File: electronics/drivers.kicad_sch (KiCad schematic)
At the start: 37 parts, among them J10 Conn_01x02_Pin, J12 GND, J13 Conn_01x08_Pin, J14 IOLV / VIO, J8 VMOT, J9 BP_MOTOR_ENABLE, Q2 PMOS_GDS, U10 ISO7762DBQ, U11 LM1117DT-3.3, U12 SFH617A-1, U8 SFH617A-1, U9 74LVC125

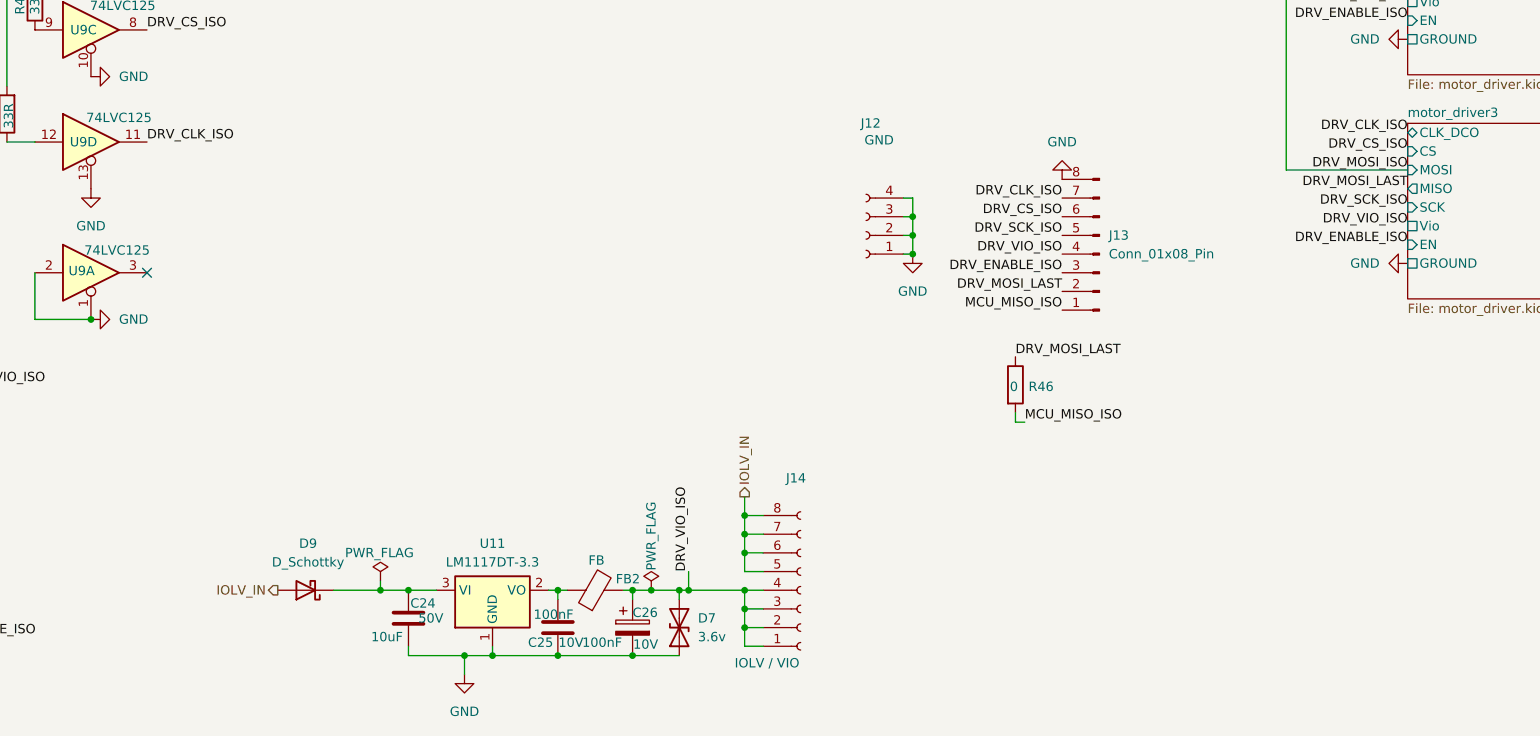
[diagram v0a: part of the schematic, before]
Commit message: Updating electronics CAD post-production
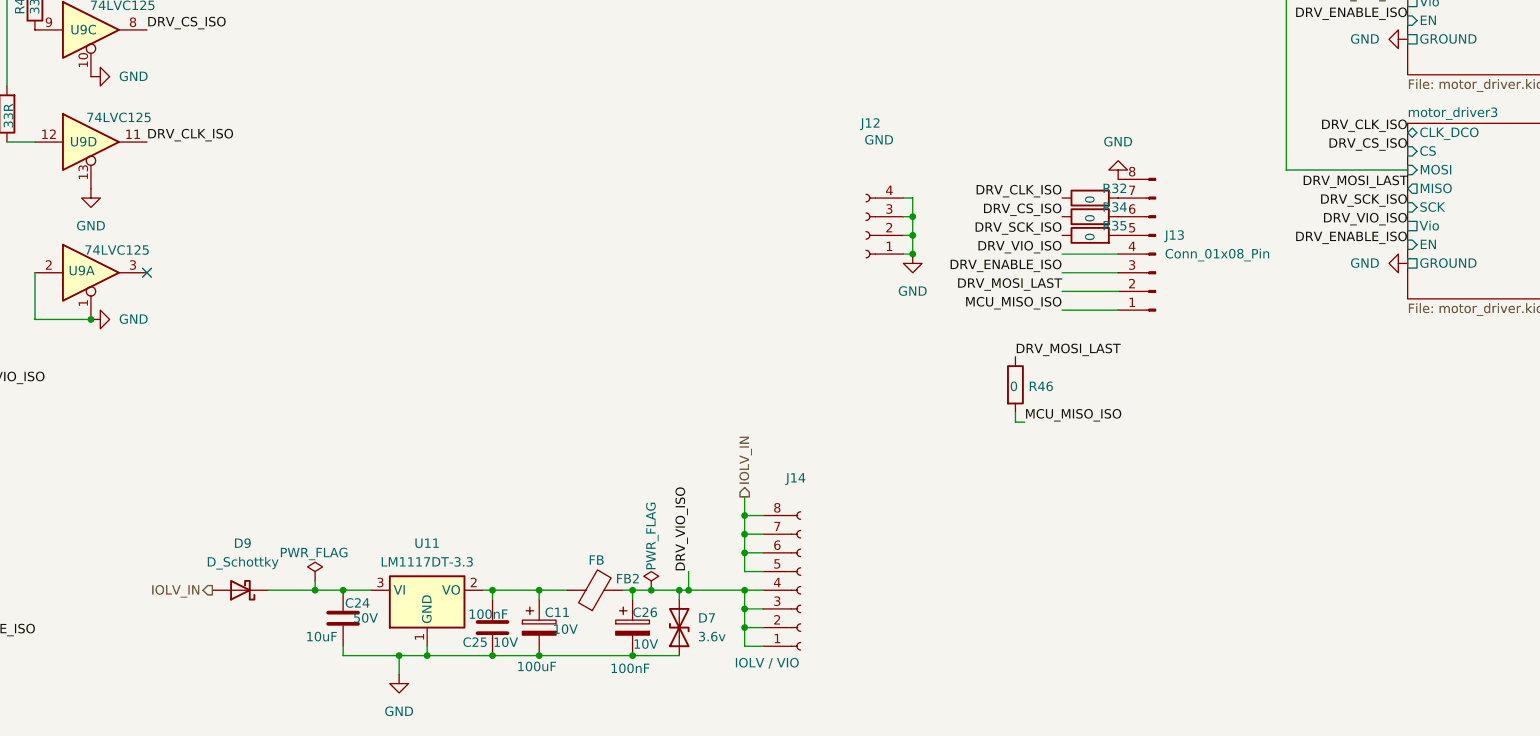
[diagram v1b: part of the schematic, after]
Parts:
- added C11: 100uF, Capacitor_THT:CP_Radial_D6.3mm_P2.50mm, symbol Device:C_Polarized
- added R32, R34, R35: 0, Jumper:SolderJumper-2_P1.3mm_Open_Pad1.0x1.5mm, symbol Device:R
- D5, D9: footprint Diode_THT:D_DO-201AD_P3.81mm_Vertical_AnodeUp -> Diode_THT:D_DO-201AD_P5.08mm_Vertical_KathodeUp
- D8: footprint Diode_THT:D_DO-41_SOD81_P2.54mm_Vertical_AnodeUp -> Diode_THT:D_DO-201AD_P5.08mm_Vertical_KathodeUp
- R41, R47: footprint Resistor_THT:R_Axial_DIN0204_L3.6mm_D1.6mm_P1.90mm_Vertical -> Resistor_THT:R_Axial_DIN0204_L3.6mm_D1.6mm_P2.54mm_Vertical
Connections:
- net DRV_CLK_ISO: now also R32.1; no longer J13.7 (Pin_7)
- net DRV_CS_ISO: now also R34.1; no longer J13.6 (Pin_6)
- net DRV_SCK_ISO: now also R35.1; no longer J13.5 (Pin_5)
- net GND: now also C11.2
- net at C25.1, FB2.1, U11.2 (VO): now also C11.1
- new net: J13.5 (Pin_5), R35.2
- new net: J13.6 (Pin_6), R34.2
- new net: J13.7 (Pin_7), R32.2
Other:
- moved on the sheet: C24, C25, D9, J13, U11
